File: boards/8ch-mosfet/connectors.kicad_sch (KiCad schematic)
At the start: 10 parts, among them J1 N2K, J2 I2C

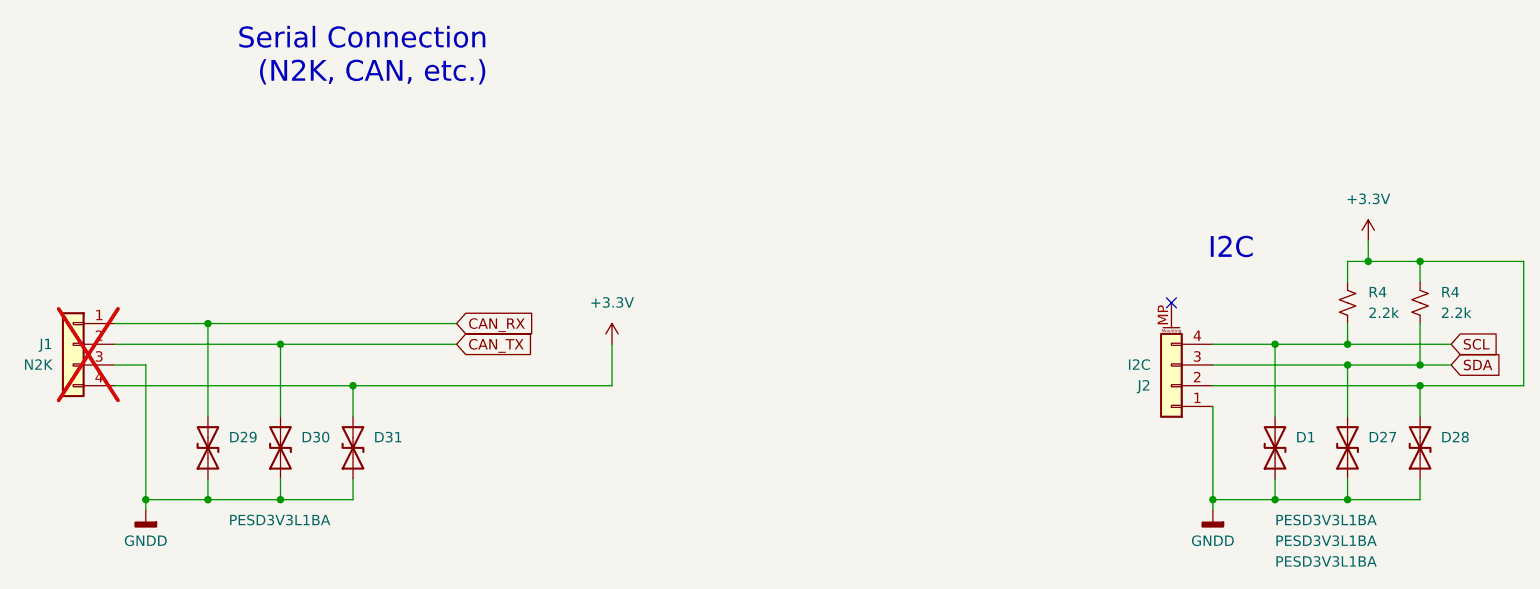
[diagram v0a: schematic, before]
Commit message: reannotated
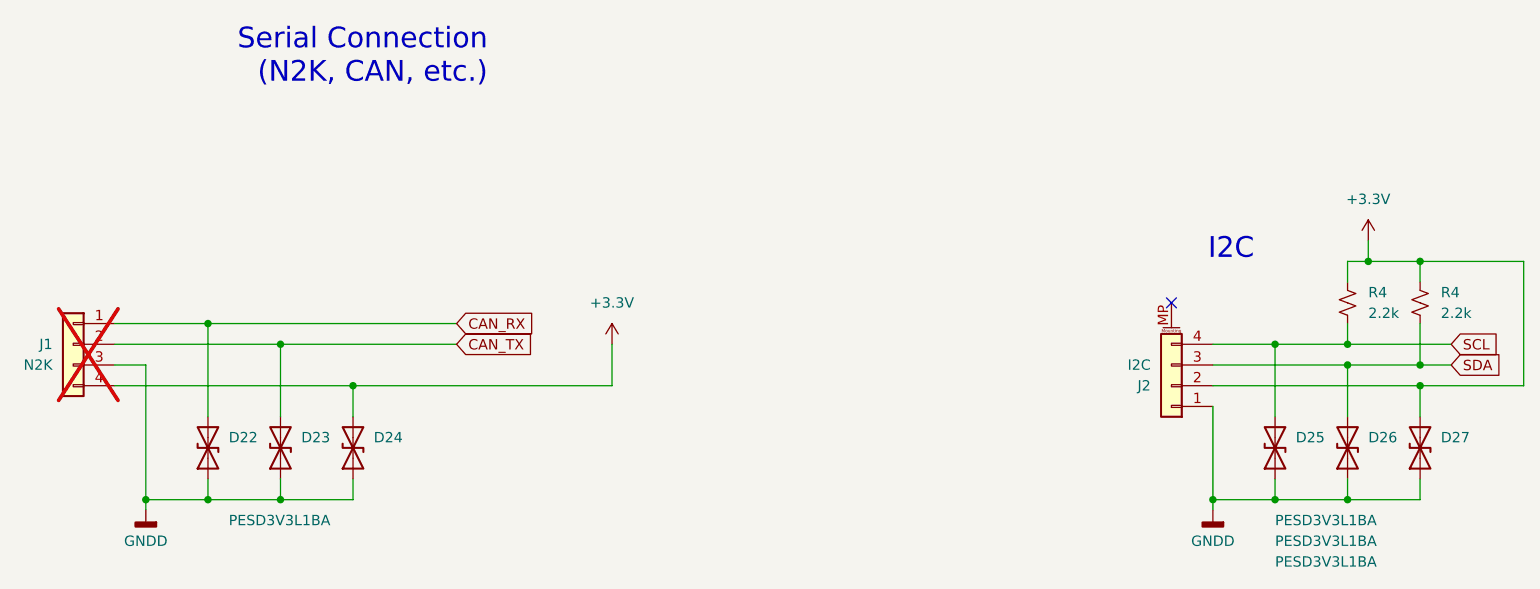
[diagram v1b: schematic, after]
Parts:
- renumbered D29 to D22, D30 to D23, D31 to D24, D1 to D25, D27 to D26, D28 to D27
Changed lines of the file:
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@@
   (symbol (lib_id "Device:D_TVS") (at 60.96 93.98 90) (unit 1)
     (in_bom yes) (on_board yes) (dnp no)
-    (property "Reference" "D30" (at 63.5 92.71 90)
+    (property "Reference" "D23" (at 63.5 92.71 90)
       (effects (font (size 1.27 1.27)) (justify right))
     )
@@
       (project "8ch-mosfet"
         (path "/c83c6236-96e9-46ad-9d7a-9e2efa4a7966/0036d08f-39b5-4a29-8e4d-ea832b2cc879"
-          (reference "D30") (unit 1)
+          (reference "D23") (unit 1)
         )
       )
@@
   (symbol (lib_id "Device:D_TVS") (at 52.07 93.98 90) (unit 1)
     (in_bom yes) (on_board yes) (dnp no)
-    (property "Reference" "D29" (at 54.61 92.71 90)
+    (property "Reference" "D22" (at 54.61 92.71 90)
       (effects (font (size 1.27 1.27)) (justify right))
     )
@@
       (project "8ch-mosfet"
         (path "/c83c6236-96e9-46ad-9d7a-9e2efa4a7966/0036d08f-39b5-4a29-8e4d-ea832b2cc879"
-          (reference "D29") (unit 1)
+          (reference "D22") (unit 1)
         )
       )
@@
         )
         (path "/c83c6236-96e9-46ad-9d7a-9e2efa4a7966/0036d08f-39b5-4a29-8e4d-ea832b2cc879"
-          (reference "J14") (unit 1)
+          (reference "J9") (unit 1)
         )
       )
@@
   (symbol (lib_id "Device:D_TVS") (at 200.66 93.98 90) (unit 1)
     (in_bom yes) (on_board yes) (dnp no)
-    (property "Reference" "D28" (at 203.2 92.71 90)
+    (property "Reference" "D27" (at 203.2 92.71 90)
       (effects (font (size 1.27 1.27)) (justify right))
     )
@@
       (project "8ch-mosfet"
         (path "/c83c6236-96e9-46ad-9d7a-9e2efa4a7966/0036d08f-39b5-4a29-8e4d-ea832b2cc879"
-          (reference "D28") (unit 1)
+          (reference "D27") (unit 1)
         )
       )
@@
   (symbol (lib_id "Device:D_TVS") (at 182.88 93.98 90) (unit 1)
     (in_bom yes) (on_board yes) (dnp no)
-    (property "Reference" "D1" (at 185.42 92.71 90)
+    (property "Reference" "D25" (at 185.42 92.71 90)
       (effects (font (size 1.27 1.27)) (justify right))
     )
@@
       (project "8ch-mosfet"
         (path "/c83c6236-96e9-46ad-9d7a-9e2efa4a7966/0036d08f-39b5-4a29-8e4d-ea832b2cc879"
-          (reference "D1") (unit 1)
+          (reference "D25") (unit 1)
         )
       )
@@
         )
         (path "/c83c6236-96e9-46ad-9d7a-9e2efa4a7966/0036d08f-39b5-4a29-8e4d-ea832b2cc879"
-          (reference "#PWR054") (unit 1)
+          (reference "#PWR057") (unit 1)
         )
       )
@@
         )
         (path "/c83c6236-96e9-46ad-9d7a-9e2efa4a7966/0036d08f-39b5-4a29-8e4d-ea832b2cc879"
-          (reference "#PWR062") (unit 1)
+          (reference "#PWR059") (unit 1)
         )
       )
@@
         )
         (path "/c83c6236-96e9-46ad-9d7a-9e2efa4a7966/0036d08f-39b5-4a29-8e4d-ea832b2cc879"
-          (reference "J13") (unit 1)
+          (reference "J10") (unit 1)
         )
       )
@@
         )
         (path "/c83c6236-96e9-46ad-9d7a-9e2efa4a7966/0036d08f-39b5-4a29-8e4d-ea832b2cc879"
-          (reference "R42") (unit 1)
+          (reference "R32") (unit 1)
         )
       )
@@
         )
         (path "/c83c6236-96e9-46ad-9d7a-9e2efa4a7966/0036d08f-39b5-4a29-8e4d-ea832b2cc879"
-          (reference "#PWR061") (unit 1)
+          (reference "#PWR060") (unit 1)
         )
       )
@@
         )
         (path "/c83c6236-96e9-46ad-9d7a-9e2efa4a7966/0036d08f-39b5-4a29-8e4d-ea832b2cc879"
-          (reference "R40") (unit 1)
+          (reference "R31") (unit 1)
         )
       )
@@
   (symbol (lib_id "Device:D_TVS") (at 191.77 93.98 90) (unit 1)
     (in_bom yes) (on_board yes) (dnp no)
-    (property "Reference" "D27" (at 194.31 92.71 90)
+    (property "Reference" "D26" (at 194.31 92.71 90)
       (effects (font (size 1.27 1.27)) (justify right))
     )
@@
       (project "8ch-mosfet"
         (path "/c83c6236-96e9-46ad-9d7a-9e2efa4a7966/0036d08f-39b5-4a29-8e4d-ea832b2cc879"
-          (reference "D27") (unit 1)
+          (reference "D26") (unit 1)
         )
       )
@@
         )
         (path "/c83c6236-96e9-46ad-9d7a-9e2efa4a7966/0036d08f-39b5-4a29-8e4d-ea832b2cc879"
-          (reference "#PWR081") (unit 1)
+          (reference "#PWR058") (unit 1)
         )
       )
@@
   (symbol (lib_id "Device:D_TVS") (at 69.85 93.98 90) (unit 1)
     (in_bom yes) (on_board yes) (dnp no)
-    (property "Reference" "D31" (at 72.39 92.71 90)
+    (property "Reference" "D24" (at 72.39 92.71 90)
       (effects (font (size 1.27 1.27)) (justify right))
     )
@@
       (project "8ch-mosfet"
         (path "/c83c6236-96e9-46ad-9d7a-9e2efa4a7966/0036d08f-39b5-4a29-8e4d-ea832b2cc879"
-          (reference "D31") (unit 1)
-        )
-      )
+          (reference "D24") (unit 1)
+        )
+      )

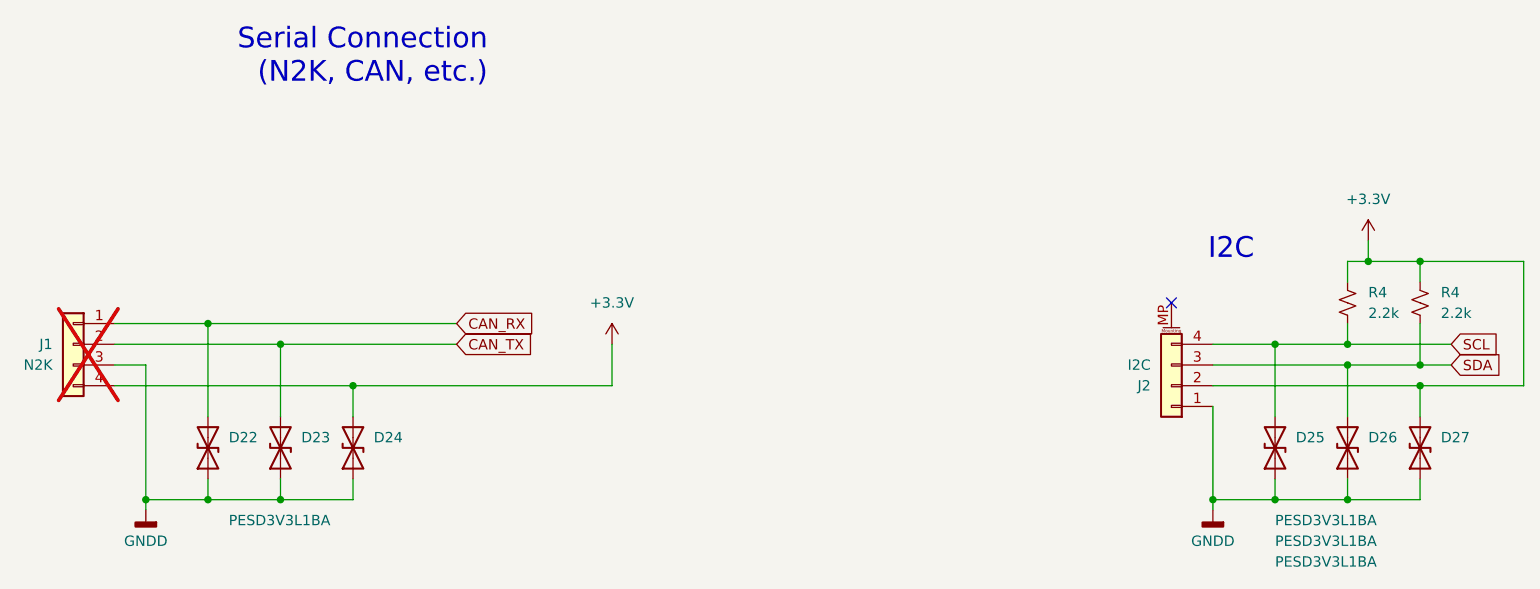
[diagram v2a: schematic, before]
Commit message: first commit of the 'totem pole' driver design
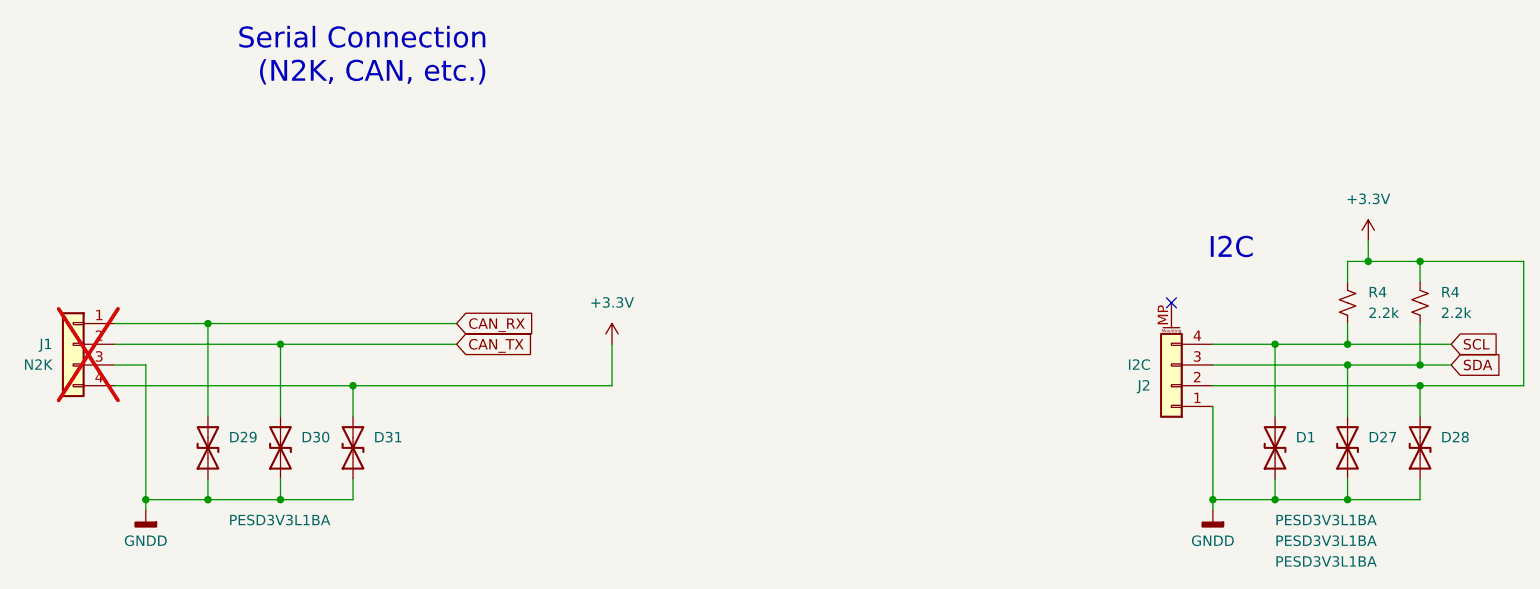
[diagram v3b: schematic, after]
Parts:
- renumbered D25 to D1, D26 to D27, D27 to D28, D22 to D29, D23 to D30, D24 to D31
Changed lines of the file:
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@@
   (title_block
     (title "Yarrboard 8ch Mosfet Driver")
-    (rev "C")
     (company "https://github.com/hoeken/yarrboard")
   )
@@
   (symbol (lib_id "Device:D_TVS") (at 60.96 93.98 90) (unit 1)
     (in_bom yes) (on_board yes) (dnp no)
-    (property "Reference" "D23" (at 63.5 92.71 90)
+    (property "Reference" "D30" (at 63.5 92.71 90)
       (effects (font (size 1.27 1.27)) (justify right))
     )
@@
       (project "8ch-mosfet"
         (path "/c83c6236-96e9-46ad-9d7a-9e2efa4a7966/0036d08f-39b5-4a29-8e4d-ea832b2cc879"
-          (reference "D23") (unit 1)
+          (reference "D30") (unit 1)
         )
       )
@@
   (symbol (lib_id "Device:D_TVS") (at 52.07 93.98 90) (unit 1)
     (in_bom yes) (on_board yes) (dnp no)
-    (property "Reference" "D22" (at 54.61 92.71 90)
+    (property "Reference" "D29" (at 54.61 92.71 90)
       (effects (font (size 1.27 1.27)) (justify right))
     )
@@
       (project "8ch-mosfet"
         (path "/c83c6236-96e9-46ad-9d7a-9e2efa4a7966/0036d08f-39b5-4a29-8e4d-ea832b2cc879"
-          (reference "D22") (unit 1)
+          (reference "D29") (unit 1)
         )
       )
@@
         )
         (path "/c83c6236-96e9-46ad-9d7a-9e2efa4a7966/0036d08f-39b5-4a29-8e4d-ea832b2cc879"
-          (reference "J9") (unit 1)
+          (reference "J14") (unit 1)
         )
       )
@@
   (symbol (lib_id "Device:D_TVS") (at 200.66 93.98 90) (unit 1)
     (in_bom yes) (on_board yes) (dnp no)
-    (property "Reference" "D27" (at 203.2 92.71 90)
+    (property "Reference" "D28" (at 203.2 92.71 90)
       (effects (font (size 1.27 1.27)) (justify right))
     )
@@
       (project "8ch-mosfet"
         (path "/c83c6236-96e9-46ad-9d7a-9e2efa4a7966/0036d08f-39b5-4a29-8e4d-ea832b2cc879"
-          (reference "D27") (unit 1)
+          (reference "D28") (unit 1)
         )
       )
@@
   (symbol (lib_id "Device:D_TVS") (at 182.88 93.98 90) (unit 1)
     (in_bom yes) (on_board yes) (dnp no)
-    (property "Reference" "D25" (at 185.42 92.71 90)
+    (property "Reference" "D1" (at 185.42 92.71 90)
       (effects (font (size 1.27 1.27)) (justify right))
     )
@@
       (project "8ch-mosfet"
         (path "/c83c6236-96e9-46ad-9d7a-9e2efa4a7966/0036d08f-39b5-4a29-8e4d-ea832b2cc879"
-          (reference "D25") (unit 1)
+          (reference "D1") (unit 1)
         )
       )
@@
         )
         (path "/c83c6236-96e9-46ad-9d7a-9e2efa4a7966/0036d08f-39b5-4a29-8e4d-ea832b2cc879"
-          (reference "#PWR057") (unit 1)
+          (reference "#PWR054") (unit 1)
         )
       )
@@
         )
         (path "/c83c6236-96e9-46ad-9d7a-9e2efa4a7966/0036d08f-39b5-4a29-8e4d-ea832b2cc879"
-          (reference "#PWR059") (unit 1)
+          (reference "#PWR062") (unit 1)
         )
       )
@@
         )
         (path "/c83c6236-96e9-46ad-9d7a-9e2efa4a7966/0036d08f-39b5-4a29-8e4d-ea832b2cc879"
-          (reference "J10") (unit 1)
+          (reference "J13") (unit 1)
         )
       )
@@
         )
         (path "/c83c6236-96e9-46ad-9d7a-9e2efa4a7966/0036d08f-39b5-4a29-8e4d-ea832b2cc879"
-          (reference "R32") (unit 1)
+          (reference "R42") (unit 1)
         )
       )
@@
         )
         (path "/c83c6236-96e9-46ad-9d7a-9e2efa4a7966/0036d08f-39b5-4a29-8e4d-ea832b2cc879"
-          (reference "#PWR060") (unit 1)
+          (reference "#PWR061") (unit 1)
         )
       )
@@
         )
         (path "/c83c6236-96e9-46ad-9d7a-9e2efa4a7966/0036d08f-39b5-4a29-8e4d-ea832b2cc879"
-          (reference "R31") (unit 1)
+          (reference "R40") (unit 1)
         )
       )
@@
   (symbol (lib_id "Device:D_TVS") (at 191.77 93.98 90) (unit 1)
     (in_bom yes) (on_board yes) (dnp no)
-    (property "Reference" "D26" (at 194.31 92.71 90)
+    (property "Reference" "D27" (at 194.31 92.71 90)
       (effects (font (size 1.27 1.27)) (justify right))
     )
@@
       (project "8ch-mosfet"
         (path "/c83c6236-96e9-46ad-9d7a-9e2efa4a7966/0036d08f-39b5-4a29-8e4d-ea832b2cc879"
-          (reference "D26") (unit 1)
+          (reference "D27") (unit 1)
         )
       )
@@
         )
         (path "/c83c6236-96e9-46ad-9d7a-9e2efa4a7966/0036d08f-39b5-4a29-8e4d-ea832b2cc879"
-          (reference "#PWR058") (unit 1)
+          (reference "#PWR081") (unit 1)
         )
       )
@@
   (symbol (lib_id "Device:D_TVS") (at 69.85 93.98 90) (unit 1)
     (in_bom yes) (on_board yes) (dnp no)
-    (property "Reference" "D24" (at 72.39 92.71 90)
+    (property "Reference" "D31" (at 72.39 92.71 90)
       (effects (font (size 1.27 1.27)) (justify right))
     )
@@
       (project "8ch-mosfet"
         (path "/c83c6236-96e9-46ad-9d7a-9e2efa4a7966/0036d08f-39b5-4a29-8e4d-ea832b2cc879"
-          (reference "D24") (unit 1)
-        )
-      )
+          (reference "D31") (unit 1)
+        )
+      )
